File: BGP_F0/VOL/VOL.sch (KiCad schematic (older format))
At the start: 4 parts, among them J1 Conn_01x03_Female, J2 Conn_01x03_Female, P1 CONN_01X02

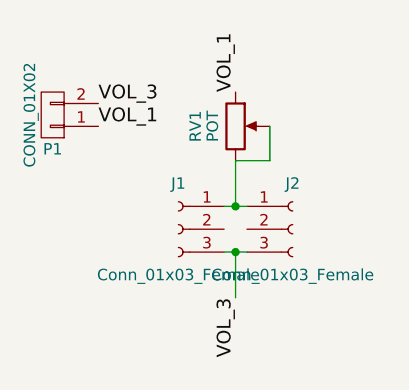
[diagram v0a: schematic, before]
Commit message: Various
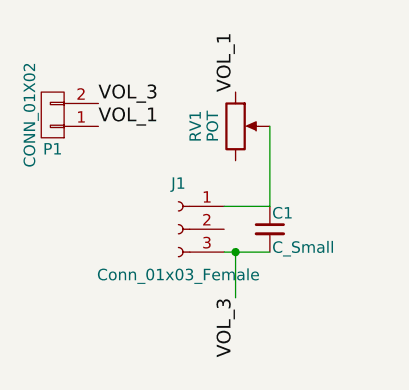
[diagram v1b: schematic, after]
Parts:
- removed J2: Conn_01x03_Female, Pin_Headers:Pin_Header_Straight_1x03_Pitch2.54mm, symbol Conn_01x03_Female
- added C1: C_Small, Capacitor_THT:C_Rect_L7.2mm_W3.0mm_P5.00mm_FKS2_FKP2_MKS2_MKP2, symbol C_Small
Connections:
- net VOL_3: now also C1.2
- net at J1.1 (Pin_1), RV1.2: now also C1.1; no longer RV1.3
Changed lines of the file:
@@
 EESchema Schematic File Version 2
+LIBS:VOL-rescue
 LIBS:power
 LIBS:device
 LIBS:switches
 LIBS:relays
-LIBS:motors
 LIBS:transistors
 LIBS:conn
@@
 $EndComp
 $Comp
-L Conn_01x03_Female J2
-U 1 1 5A7FCBD4
-P 6050 3650
-F 0 "J2" H 6050 3850 50  0000 C CNN
-F 1 "Conn_01x03_Female" H 6050 3450 50  0000 C CNN
-F 2 "Pin_Headers:Pin_Header_Straight_1x03_Pitch2.54mm" H 6050 3650 50  0001 C CNN
-F 3 "" H 6050 3650 50  0001 C CNN
-	1    6050 3650
-	1    0    0    -1
-$EndComp
-$Comp
 L Conn_01x03_Female J1
 U 1 1 5A7FCBFC
@@
 $EndComp
 Wire Wire Line
-	5800 3350 5800 3550
+	5800 3750 5800 3950
 Wire Wire Line
-	5750 3550 5850 3550
-Connection ~ 5800 3550
+	5950 3550 5950 3200
 Wire Wire Line
-	5750 3750 5850 3750
+	5750 3550 5950 3550
 Wire Wire Line
-	5800 3750 5800 3950
+	5750 3750 5950 3750
+$Comp
+L C_Small C1
+U 1 1 5AF91950
+P 5950 3650
+F 0 "C1" H 5960 3720 50  0000 L CNN
+F 1 "C_Small" H 5960 3570 50  0000 L CNN
+F 2 "Capacitor_THT:C_Rect_L7.2mm_W3.0mm_P5.00mm_FKS2_FKP2_MKS2_MKP2" H 5950 3650 50  0001 C CNN
+F 3 "" H 5950 3650 50  0000 C CNN
+	1    5950 3650
+	1    0    0    -1
+$EndComp
 Connection ~ 5800 3750
-Wire Wire Line
-	5950 3200 5950 3350
-Wire Wire Line
-	5950 3350 5800 3350
 $EndSCHEMATC
